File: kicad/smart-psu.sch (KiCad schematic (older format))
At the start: 21 parts, among them J1 DC-IN, J2 Conn_01x03, J3 Conn_01x03, Q1 TUP, Q2 P2003ED, SW1 SW_DIP_x02, U1 LM2596S-5, U2 AP1117-33, U3 ATtiny13A-PU

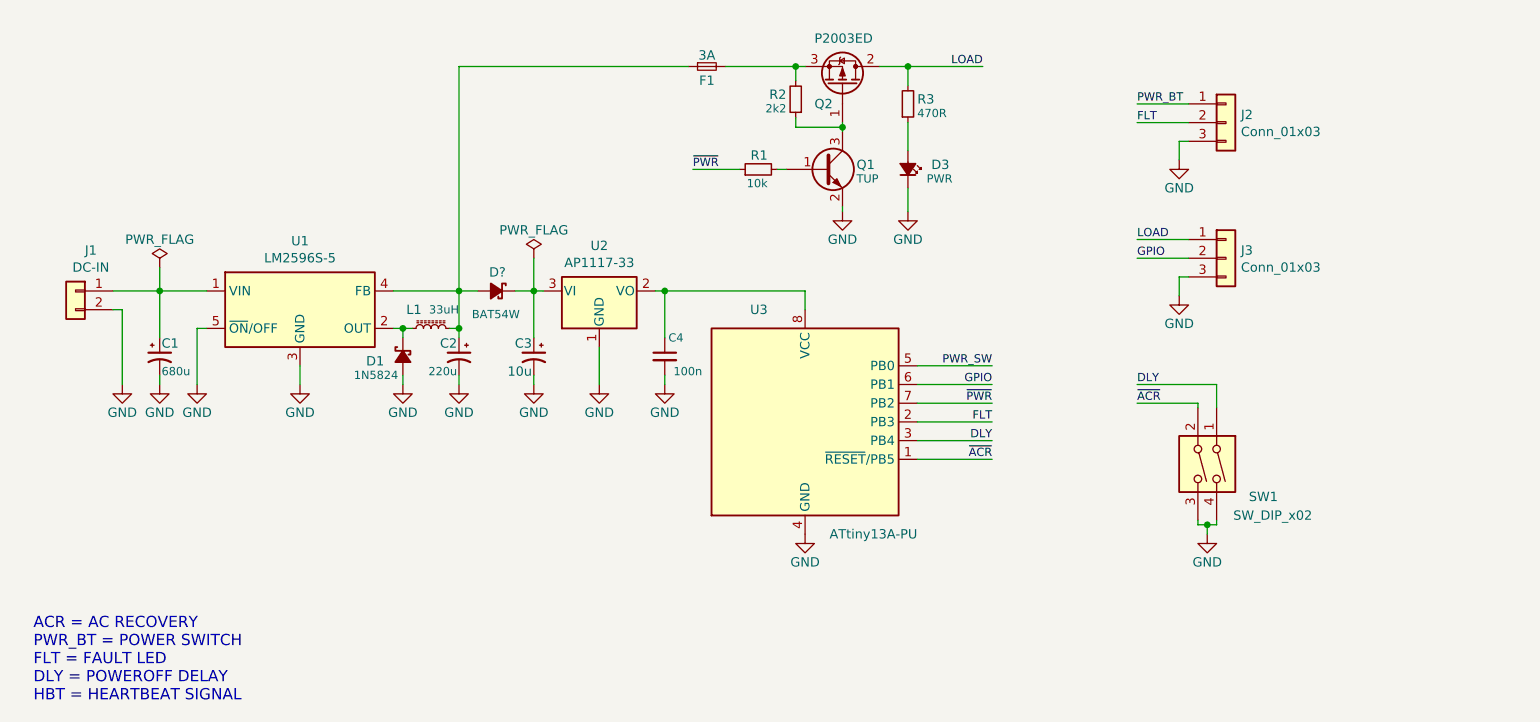
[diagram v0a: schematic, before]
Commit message: Update schematic
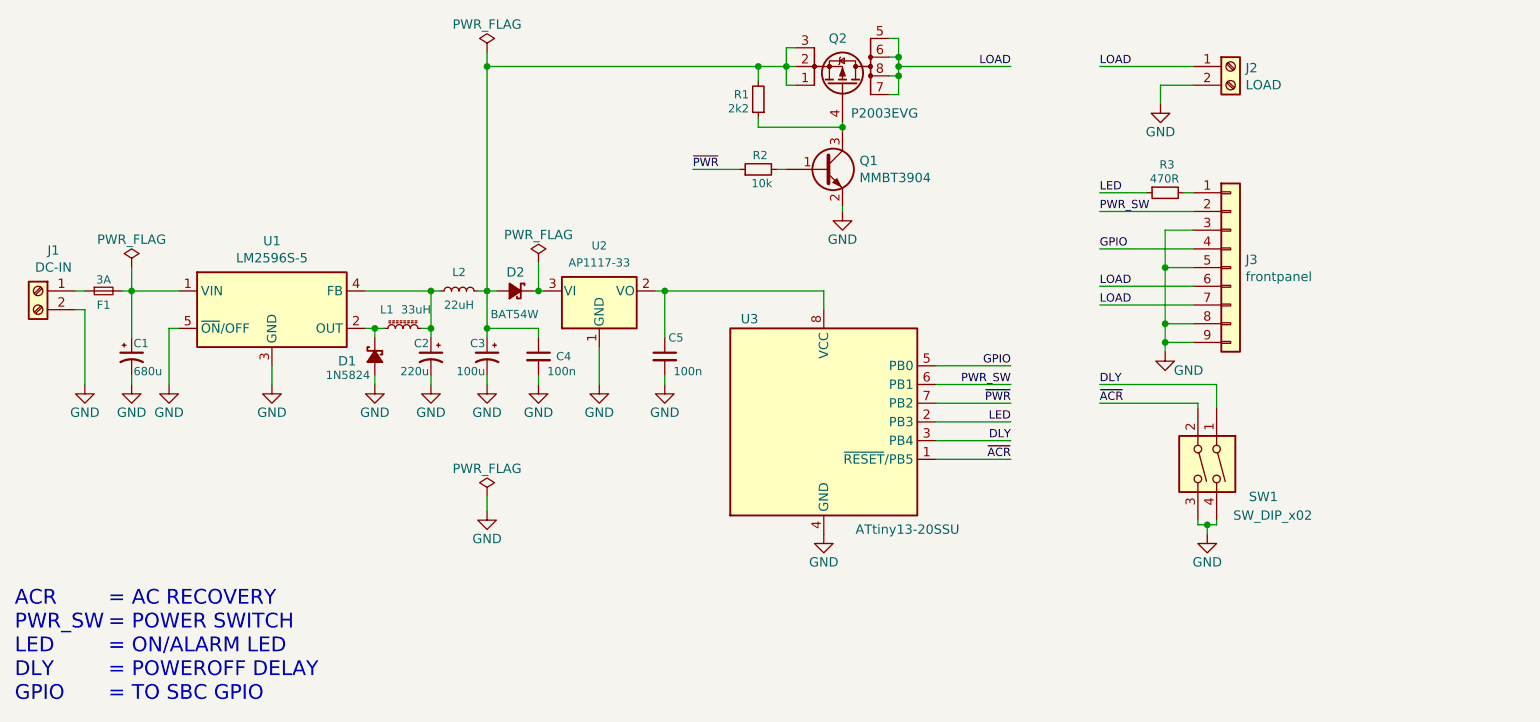
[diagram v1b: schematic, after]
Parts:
- removed D3: PWR, symbol Device:LED_Small_ALT
- removed J1: DC-IN, symbol Connector_Generic:Conn_01x02
- removed J2, J3: Conn_01x03, symbol Connector_Generic:Conn_01x03
- removed Q1: TUP, symbol Device:Q_NPN_BEC
- removed Q2: P2003ED, symbol Device:Q_PMOS_GDS
- removed U3: ATtiny13A-PU, Package_DIP:DIP-8_W7.62mm, symbol MCU_Microchip_ATtiny:ATtiny13A-PU
- added C4: 100n, Capacitor_SMD:C_1206_3216Metric_Pad1.33x1.80mm_HandSolder, symbol Device:C_Small
- added J1: DC-IN, TerminalBlock_MetzConnect:TerminalBlock_MetzConnect_Type055_RT01502HDWU_1x02_P5.00mm_Horizontal, symbol Connector:Screw_Terminal_01x02
- added J2: LOAD, TerminalBlock_MetzConnect:TerminalBlock_MetzConnect_Type055_RT01502HDWU_1x02_P5.00mm_Horizontal, symbol Connector:Screw_Terminal_01x02
- added J3: frontpanel, Connector_PinHeader_2.54mm:PinHeader_1x09_P2.54mm_Vertical, symbol Connector_Generic:Conn_01x09
- added L2: 22uH, Inductor_THT:L_Toroid_Vertical_L21.6mm_W11.4mm_P7.62mm_Pulse_KM-3, symbol Device:L_Small
- added Q1: MMBT3904, Package_TO_SOT_SMD:SOT-23, symbol Transistor_BJT:MMBT3904
- added Q2: P2003EVG, Package_SO:SOIC-8_3.9x4.9mm_P1.27mm, symbol Transistor_FET:P2003EVG
- added U3: ATtiny13-20SSU, Package_SO:SOIC-8_3.9x4.9mm_P1.27mm, symbol MCU_Microchip_ATtiny:ATtiny13-20SSU
- C1: footprint Capacitors_THT:CP_Radial_D10.0mm_P5.00mm_P7.50mm -> Capacitor_THT:C_Radial_D10.0mm_H20.0mm_P5.00mm
- C2: footprint Capacitors_THT:CP_Radial_D8.0mm_P3.50mm -> Capacitor_THT:CP_Radial_D8.0mm_P2.50mm
- C3: value 10u -> 100u; footprint Capacitors_THT:CP_Radial_D7.5mm_P2.50mm -> Capacitor_THT:CP_Radial_D5.0mm_P2.50mm
- C5: renamed from C4; footprint Capacitors_SMD:C_1206_HandSoldering -> Capacitor_SMD:C_1206_3216Metric_Pad1.33x1.80mm_HandSolder
- D1: footprint (none) -> Diode_THT:D_A-405_P12.70mm_Horizontal
- D2: renamed from D?; footprint (none) -> Diode_SMD:D_1206_3216Metric_Pad1.42x1.75mm_HandSolder
- F1: footprint SMD_Packages:SMD-1206_Pol -> Fuse:Fuse_1206_3216Metric_Pad1.42x1.75mm_HandSolder
- L1: footprint Choke_Toroid_ThroughHole:Choke_Toroid_6,5x13mm_Vertical -> Inductor_THT:L_Toroid_Vertical_L21.6mm_W11.4mm_P7.62mm_Pulse_KM-3
- R1: renamed from R2; footprint Resistor_SMD:R_1206_3216Metric_Pad1.42x1.75mm_HandSolder -> Resistor_SMD:R_1206_3216Metric_Pad1.30x1.75mm_HandSolder
- R2: renamed from R1; footprint Resistor_SMD:R_1206_3216Metric_Pad1.42x1.75mm_HandSolder -> Resistor_SMD:R_1206_3216Metric_Pad1.30x1.75mm_HandSolder
- R3: footprint Resistor_SMD:R_1206_3216Metric_Pad1.42x1.75mm_HandSolder -> Resistor_SMD:R_1206_3216Metric_Pad1.30x1.75mm_HandSolder
- SW1: footprint (none) -> Button_Switch_THT:SW_DIP_SPSTx02_Slide_9.78x7.26mm_W7.62mm_P2.54mm
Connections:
- net DLY: now also U3.3 (PB4)
- net GND: now also C4.2, J1.2 (Pin_2), J2.2 (Pin_2), J3.3 (Pin_3), J3.5 (Pin_5), J3.8 (Pin_8), J3.9 (Pin_9), Q1.2 (E), U3.4 (GND)
- net GPIO: now also J3.4 (Pin_4), U3.5 (PB0)
- net LOAD: now also J2.1 (Pin_1), J3.6 (Pin_6), J3.7 (Pin_7), Q2.5 (D), Q2.6 (D), Q2.7 (D), Q2.8 (D); no longer R3.2
- net PWR_SW: now also J3.2 (Pin_2), U3.6 (PB1)
- net ~ACR: now also U3.1 (~RESET~/PB5)
- net ~PWR: now also U3.7 (PB2)
- net at C2.1, L1.2, U1.4 (FB): now also L2.2; no longer D2.2 (A), F1.1
- net at F1.2: now also C1.1, U1.1 (VIN); no longer R1.2
- net LED: now reaches R3.1
- net LED: now also U3.2 (PB3)
- net at R1.1: now also Q1.3 (C), Q2.4 (G)
- net at R2.2: now also Q1.1 (B)
- net at C5.1, U2.2 (VO): now also U3.8 (VCC)
- net at D2.1 (K), U2.3 (VI): no longer C3.1
- new net: F1.1, J1.1 (Pin_1)
- new net: J3.1 (Pin_1), R3.2
- new net: C3.1, C4.1, D2.2 (A), L2.1, Q2.1 (S), Q2.2 (S), Q2.3 (S), R1.2
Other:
- note added: "= AC RECOVERY\n= POWER SWITCH\n= ON/ALARM LED\n= POWEROFF DELAY\n= TO SBC GPIO"
- note added: "ACR \nPWR_SW \nLED \nDLY\nGPIO"
- note removed: "ACR = AC RECOVERY\nPWR_BT = POWER SWITCH\nFLT = FAULT LED\nDLY = POWEROFF DELAY\nHBT = HEARTBEAT SIGNAL"
- moved on the sheet: C1, C2, C3, D1, D2, F1, L1, R1, R3, U1

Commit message: Update frontpanel connector
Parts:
- removed J3: frontpanel, Connector_PinHeader_2.54mm:PinHeader_1x09_P2.54mm_Vertical, symbol Connector_Generic:Conn_01x09
- added J3: frontpanel, Connector_PinHeader_2.54mm:PinHeader_2x05_P2.54mm_Vertical, symbol Connector_Generic:Conn_02x05_Odd_Even
- Q2: symbol Transistor_FET:P2003EVG -> smart-psu-rescue:P2003EVG-Transistor_FET
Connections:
- net GND: now also J3.10 (Pin_10), J3.2 (Pin_2), J3.4 (Pin_4), J3.6 (Pin_6), J3.9 (Pin_9)
- net GPIO: now also J3.5 (Pin_5)
- net LOAD: now also J3.7 (Pin_7), J3.8 (Pin_8)
- net PWR_SW: now also J3.3 (Pin_3)
- net at R3.2: now also J3.1 (Pin_1)
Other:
- moved on the sheet: J2, R3, SW1
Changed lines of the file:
@@
 Comment4 ""
 $EndDescr
-Text Label 7550 3900 2    44   ~ 0
-LED
 Text Label 7550 3800 2    44   ~ 0
 ~PWR
@@
 L Device:R_Small R3
 U 1 1 5AC2239F
-P 8375 2675
-F 0 "R3" V 8225 2625 44  0000 L CNN
-F 1 "470R" V 8300 2600 44  0000 L CNN
-F 2 "Resistor_SMD:R_1206_3216Metric_Pad1.30x1.75mm_HandSolder" H 8375 2675 50  0001 C CNN
-F 3 "" H 8375 2675 50  0001 C CNN
-	1    8375 2675
+P 9100 3000
+F 0 "R3" V 8950 2950 44  0000 L CNN
+F 1 "470R" V 9025 2925 44  0000 L CNN
+F 2 "Resistor_SMD:R_1206_3216Metric_Pad1.30x1.75mm_HandSolder" H 9100 3000 50  0001 C CNN
+F 3 "" H 9100 3000 50  0001 C CNN
+	1    9100 3000
 	0    -1   1    0
 $EndComp
-Text Label 8025 3700 0    44   ~ 0
+Text Label 8750 4325 0    44   ~ 0
 DLY
-Text Label 8025 3800 0    44   ~ 0
+Text Label 8750 4425 0    44   ~ 0
 ~ACR
-Text Label 8025 2000 0    44   ~ 0
+Text Label 8775 2000 0    44   ~ 0
 LOAD
 $Comp
@@
 L power:GND #PWR015
 U 1 1 5ACD42F7
-P 8600 4500
-F 0 "#PWR015" H 8600 4250 50  0001 C CNN
-F 1 "GND" H 8600 4350 50  0000 C CNN
-F 2 "" H 8600 4500 50  0000 C CNN
-F 3 "" H 8600 4500 50  0000 C CNN
-	1    8600 4500
+P 9325 5125
+F 0 "#PWR015" H 9325 4875 50  0001 C CNN
+F 1 "GND" H 9325 4975 50  0000 C CNN
+F 2 "" H 9325 5125 50  0000 C CNN
+F 3 "" H 9325 5125 50  0000 C CNN
+	1    9325 5125
 	1    0    0    -1
 $EndComp
@@
 Wire Wire Line
 	7150 4100 7550 4100
-Text Label 7550 3600 2    44   ~ 0
-GPIO
-Text Label 8025 2975 0    44   ~ 0
+Text Label 8750 3200 0    44   ~ 0
 GPIO
 $Comp
@@
 L Switch:SW_DIP_x02 SW1
 U 1 1 5C89B5F2
-P 8550 4125
-F 0 "SW1" V 8725 4475 50  0000 C CNN
-F 1 "SW_DIP_x02" V 8825 4525 50  0000 C CNN
-F 2 "Button_Switch_THT:SW_DIP_SPSTx02_Slide_9.78x7.26mm_W7.62mm_P2.54mm" H 8550 4125 50  0001 C CNN
-F 3 "" H 8550 4125 50  0001 C CNN
-	1    8550 4125
+P 9275 4750
+F 0 "SW1" V 9450 5100 50  0000 C CNN
+F 1 "SW_DIP_x02" V 9550 5150 50  0000 C CNN
+F 2 "Button_Switch_THT:SW_DIP_SPSTx02_Slide_9.78x7.26mm_W7.62mm_P2.54mm" H 9275 4750 50  0001 C CNN
+F 3 "" H 9275 4750 50  0001 C CNN
+	1    9275 4750
 	0    1    1    0
 $EndComp
@@
 L power:GND #PWR014
 U 1 1 606342F9
-P 8375 3525
-F 0 "#PWR014" H 8375 3275 50  0001 C CNN
-F 1 "GND" H 8500 3425 50  0000 C CNN
-F 2 "" H 8375 3525 50  0000 C CNN
-F 3 "" H 8375 3525 50  0000 C CNN
-	1    8375 3525
-	1    0    0    -1
-$EndComp
-Text Label 8025 2775 0    44   ~ 0
+P 9175 3500
+F 0 "#PWR014" H 9175 3250 50  0001 C CNN
+F 1 "GND" H 9300 3400 50  0000 C CNN
+F 2 "" H 9175 3500 50  0000 C CNN
+F 3 "" H 9175 3500 50  0000 C CNN
+	1    9175 3500
+	1    0    0    -1
+$EndComp
+Text Label 8750 3100 0    44   ~ 0
 PWR_SW
-Text Label 8025 2675 0    44   ~ 0
-LED
-Wire Wire Line
-	8550 4425 8550 4450
-Wire Wire Line
-	8550 4450 8600 4450
-Wire Wire Line
-	8650 4450 8650 4425
-Wire Wire Line
-	8600 4500 8600 4450
-Connection ~ 8600 4450
-Wire Wire Line
-	8600 4450 8650 4450
-Wire Wire Line
-	8550 3800 8550 3825
-Wire Wire Line
-	8650 3700 8650 3825
+Wire Wire Line
+	9275 5050 9275 5075
+Wire Wire Line
+	9275 5075 9325 5075
+Wire Wire Line
+	9375 5075 9375 5050
+Wire Wire Line
+	9325 5125 9325 5075
+Connection ~ 9325 5075
+Wire Wire Line
+	9325 5075 9375 5075
+Wire Wire Line
+	9275 4425 9275 4450
+Wire Wire Line
+	9375 4325 9375 4450
 Wire Wire Line
 	2850 3650 2850 3700
@@
 Text Notes 2725 5400 0    79   ~ 0
 = AC RECOVERY\n= POWER SWITCH\n= ON/ALARM LED\n= POWEROFF DELAY\n= TO SBC GPIO
-Wire Wire Line
-	8025 2975 8525 2975
-Wire Wire Line
-	8275 2675 8025 2675
-$Comp
-L Transistor_FET:P2003EVG Q2
+$Comp
+L smart-psu-rescue:P2003EVG-Transistor_FET Q2
 U 1 1 606660A4
 P 6650 2100
@@
 L Connector:Screw_Terminal_01x02 J2
 U 1 1 60677164
-P 8725 2000
-F 0 "J2" H 8805 1992 50  0000 L CNN
-F 1 "LOAD" H 8805 1901 50  0000 L CNN
-F 2 "TerminalBlock_MetzConnect:TerminalBlock_MetzConnect_Type055_RT01502HDWU_1x02_P5.00mm_Horizontal" H 8725 2000 50  0001 C CNN
-F 3 "~" H 8725 2000 50  0001 C CNN
-	1    8725 2000
-	1    0    0    -1
-$EndComp
-Wire Wire Line
-	8475 2675 8525 2675
-Wire Wire Line
-	8025 2775 8525 2775
+P 9475 2000
+F 0 "J2" H 9555 1992 50  0000 L CNN
+F 1 "LOAD" H 9555 1901 50  0000 L CNN
+F 2 "TerminalBlock_MetzConnect:TerminalBlock_MetzConnect_Type055_RT01502HDWU_1x02_P5.00mm_Horizontal" H 9475 2000 50  0001 C CNN
+F 3 "~" H 9475 2000 50  0001 C CNN
+	1    9475 2000
+	1    0    0    -1
+$EndComp
+Wire Wire Line
+	9200 3000 9250 3000
 $Comp
 L power:GND #PWR013
 U 1 1 6068BD21
-P 8350 2200
-F 0 "#PWR013" H 8350 1950 50  0001 C CNN
-F 1 "GND" H 8350 2050 50  0000 C CNN
-F 2 "" H 8350 2200 50  0000 C CNN
-F 3 "" H 8350 2200 50  0000 C CNN
-	1    8350 2200
-	1    0    0    -1
-$EndComp
-Text Label 8025 3175 0    44   ~ 0
+P 9100 2200
+F 0 "#PWR013" H 9100 1950 50  0001 C CNN
+F 1 "GND" H 9100 2050 50  0000 C CNN
+F 2 "" H 9100 2200 50  0000 C CNN
+F 3 "" H 9100 2200 50  0000 C CNN
+	1    9100 2200
+	1    0    0    -1
+$EndComp
+Text Label 8750 3300 0    44   ~ 0
 LOAD
-Text Label 8025 3275 0    44   ~ 0
+Text Label 10300 3300 2    44   ~ 0
 LOAD
-Wire Wire Line
-	8025 3175 8525 3175
-Wire Wire Line
-	8525 3275 8025 3275
-$Comp
-L Connector_Generic:Conn_01x09 J3
-U 1 1 606A2659
-P 8725 3075
-F 0 "J3" H 8805 3117 50  0000 L CNN
-F 1 "frontpanel" H 8805 3026 50  0000 L CNN
-F 2 "Connector_PinHeader_2.54mm:PinHeader_1x09_P2.54mm_Vertical" H 8725 3075 50  0001 C CNN
-F 3 "~" H 8725 3075 50  0001 C CNN
-	1    8725 3075
-	1    0    0    -1
-$EndComp
 $Comp
 L MCU_Microchip_ATtiny:ATtiny13-20SSU U3
@@
 	4750 3400 5025 3400
 Wire Wire Line
-	8350 2200 8350 2100
-Wire Wire Line
-	8025 2000 8525 2000
-Wire Wire Line
-	8525 2100 8350 2100
+	9100 2200 9100 2100
+Wire Wire Line
+	8775 2000 9275 2000
+Wire Wire Line
+	9275 2100 9100 2100
 Wire Wire Line
 	6550 3200 6550 3300
@@
 	6950 2000 7550 2000
 Wire Wire Line
-	8025 3700 8650 3700
-Wire Wire Line
-	8025 3800 8550 3800
-Wire Wire Line
-	8375 2875 8375 3075
-Wire Wire Line
-	8375 2875 8525 2875
-Wire Wire Line
-	8375 3075 8525 3075
-Wire Wire Line
-	8375 3075 8375 3375
-Connection ~ 8375 3075
-Wire Wire Line
-	8375 3375 8525 3375
-Connection ~ 8375 3375
-Wire Wire Line
-	8375 3375 8375 3475
-Wire Wire Line
-	8525 3475 8375 3475
-Connection ~ 8375 3475
-Wire Wire Line
-	8375 3475 8375 3525
+	8750 4325 9375 4325
+Wire Wire Line
+	8750 4425 9275 4425
+Text Label 7550 3900 2    44   ~ 0
+LED
+Text Label 7550 3600 2    44   ~ 0
+GPIO
+Wire Wire Line
+	8750 3000 9000 3000
+Text Label 8750 3000 0    44   ~ 0
+LED
+$Comp
+L Connector_Generic:Conn_02x05_Odd_Even J3
+U 1 1 618C2BC7
+P 9450 3200
+F 0 "J3" H 9500 3617 50  0000 C CNN
+F 1 "frontpanel" H 9500 3526 50  0000 C CNN
+F 2 "Connector_PinHeader_2.54mm:PinHeader_2x05_P2.54mm_Vertical" H 9450 3200 50  0001 C CNN
+F 3 "~" H 9450 3200 50  0001 C CNN
+	1    9450 3200
+	1    0    0    -1
+$EndComp
+Wire Wire Line
+	8750 3100 9250 3100
+Wire Wire Line
+	8750 3200 9250 3200
+Wire Wire Line
+	9750 3300 10300 3300
+Wire Wire Line
+	9175 3500 9175 3400
+Wire Wire Line
+	9175 3400 9250 3400
+$Comp
+L power:GND #PWR016
+U 1 1 618D87C0
+P 9850 3500
+F 0 "#PWR016" H 9850 3250 50  0001 C CNN
+F 1 "GND" H 9975 3400 50  0000 C CNN
+F 2 "" H 9850 3500 50  0000 C CNN
+F 3 "" H 9850 3500 50  0000 C CNN
+	1    9850 3500
+	1    0    0    -1
+$EndComp
+Wire Wire Line
+	9750 3400 9850 3400
+Wire Wire Line
+	9850 3400 9850 3500
+Wire Wire Line
+	9750 3000 9850 3000
+Wire Wire Line
+	9850 3000 9850 3100
+Connection ~ 9850 3400
+Wire Wire Line
+	9750 3100 9850 3100
+Connection ~ 9850 3100
+Wire Wire Line
+	9850 3100 9850 3200
+Wire Wire Line
+	8750 3300 9250 3300
+Wire Wire Line
+	9750 3200 9850 3200
+Connection ~ 9850 3200
+Wire Wire Line
+	9850 3200 9850 3400
 $EndSCHEMATC
